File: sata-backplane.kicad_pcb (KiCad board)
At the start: 2 copper layers, 100 x 60 mm, 26 parts, among them J5 457180002, J6 G40H3132212HR, U1 TPS563201DDCR, U5 TPS563201DDCR

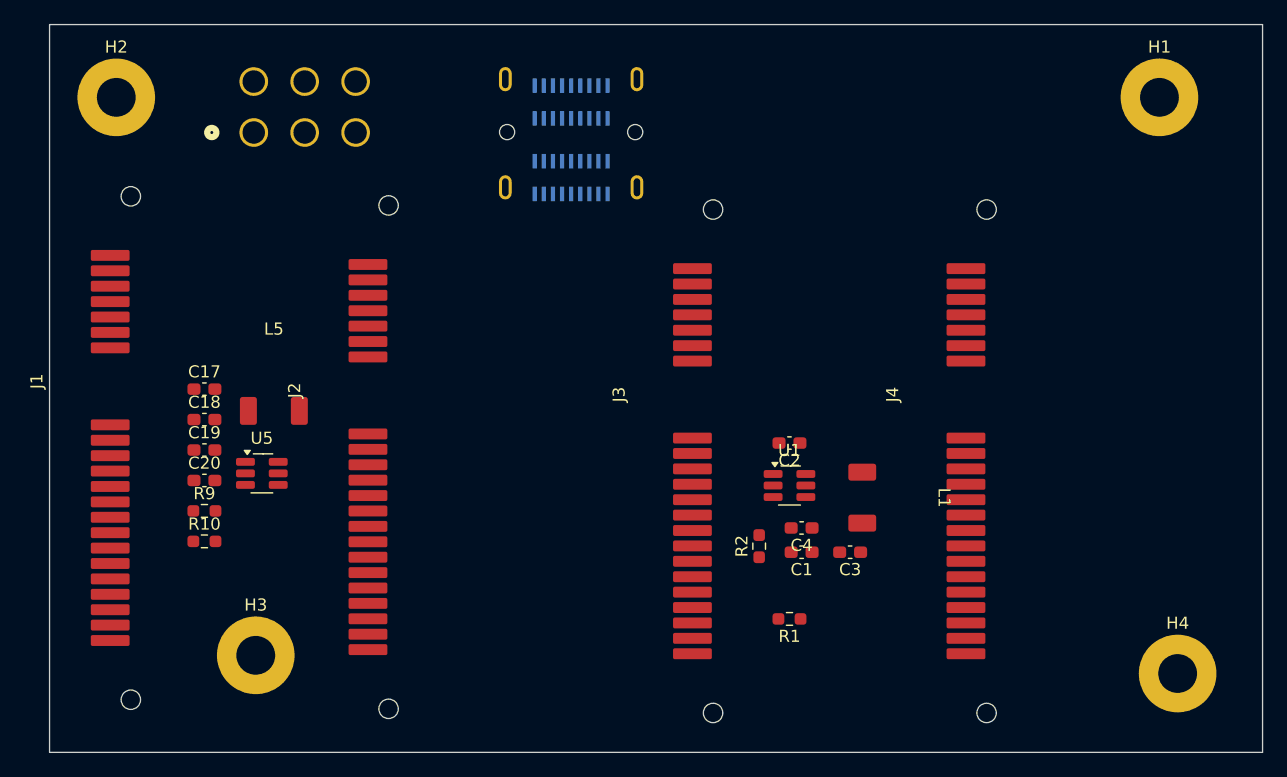
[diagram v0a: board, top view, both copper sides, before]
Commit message: Rough layout
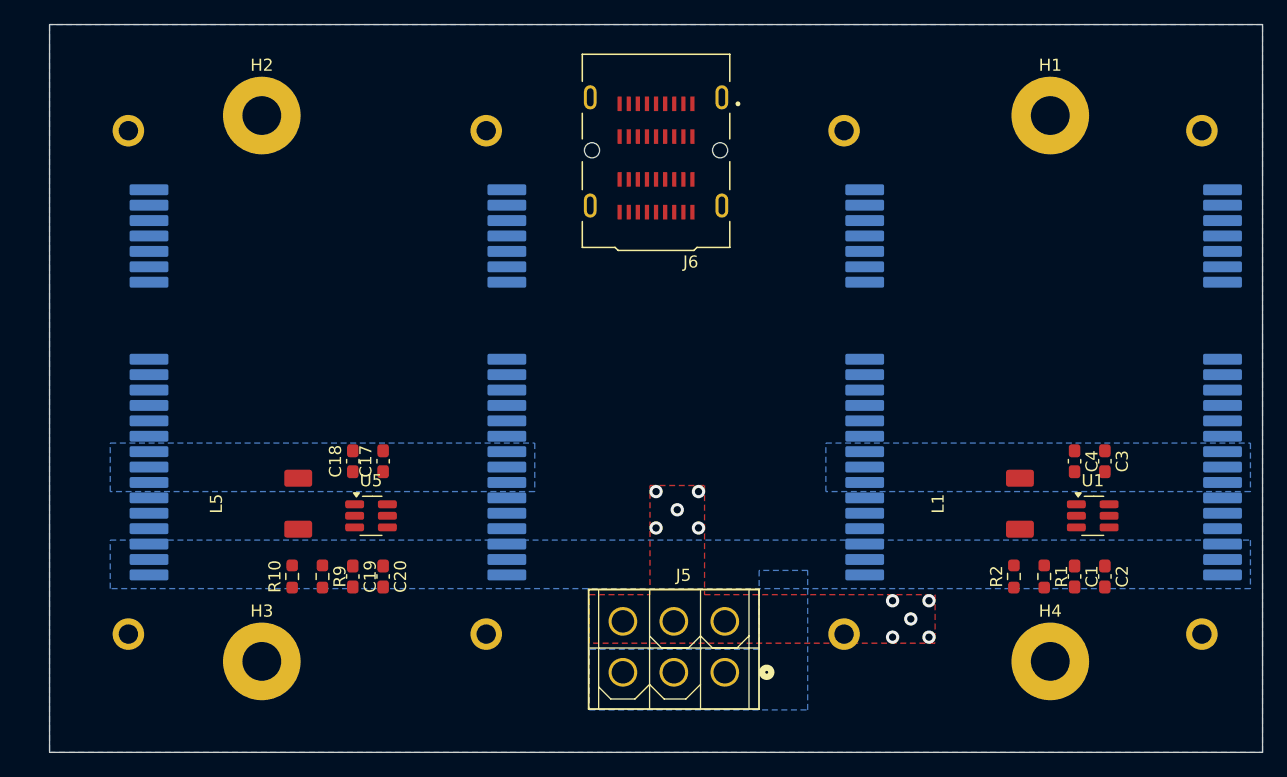
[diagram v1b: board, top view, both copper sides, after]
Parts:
- J1, J2, J3, J4: moved to B.Cu
- J5: moved to F.Cu
- J6: footprint G40H3132212HR:AMPHENOL_G40H3132212HR -> 00-Local:AMPHENOL_G40H3132212HR; moved to F.Cu
- moved J5 59.1 mm to (193.2, 120.9), turned to 0 degrees
- moved C2 28.2 mm to (224.5, 113.0), turned to -90 degrees
- moved U1 25.1 mm to (223.5, 108.0)
- moved C4 23.2 mm to (222.0, 103.5), turned to -90 degrees
- moved C1 22.6 mm to (222.0, 113.0), turned to -90 degrees
- moved C3 22.3 mm to (224.5, 103.5), turned to -90 degrees
- moved J4 21.4 mm to (234.0, 97.0)
- moved R1 21.3 mm to (219.5, 113.0), turned to -90 degrees
- moved R2 21.1 mm to (217.0, 113.0)
- moved C20 16.7 mm to (165.0, 113.0), turned to -90 degrees
- moved C19 16.1 mm to (162.5, 113.0), turned to -90 degrees
- moved C17 15.9 mm to (165.0, 103.5), turned to 90 degrees
- moved J3 14.7 mm to (204.5, 97.0)
- moved L1 13.0 mm to (217.5, 107.0), turned to 90 degrees
- moved C18 12.7 mm to (162.5, 103.5), turned to 90 degrees
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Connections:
- C1 pad 1: Net-(U1-EN) -> +12V
- C19 pad 1: Net-(U5-EN) -> +12V
- C2 pad 1: Net-(U1-EN) -> +12V
- C20 pad 1: Net-(U5-EN) -> +12V
- J5 pad 4: unconnected-(J5-Pad4) -> GND
- U1 pad 3: Net-(U1-EN) -> +12V
- U1 pad 5: Net-(U1-EN) -> +12V
- U5 pad 3: Net-(U5-EN) -> +12V
- U5 pad 5: Net-(U5-EN) -> +12V
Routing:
- net GND: vias 0 -> 10
- added copper zone on B.Cu, net +12V
- added copper zone on B.Cu, net +5V_1
- added copper zone on B.Cu, net +5V_2
- added copper zone on B.Cu, net GND
- added copper zone on F.Cu, net GND
